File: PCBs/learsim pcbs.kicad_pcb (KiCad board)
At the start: 2 copper layers, 11 parts, among them U1 ESP32-C6-DEV-KIT-N8, U2 MAX7219, U3 MAX7219

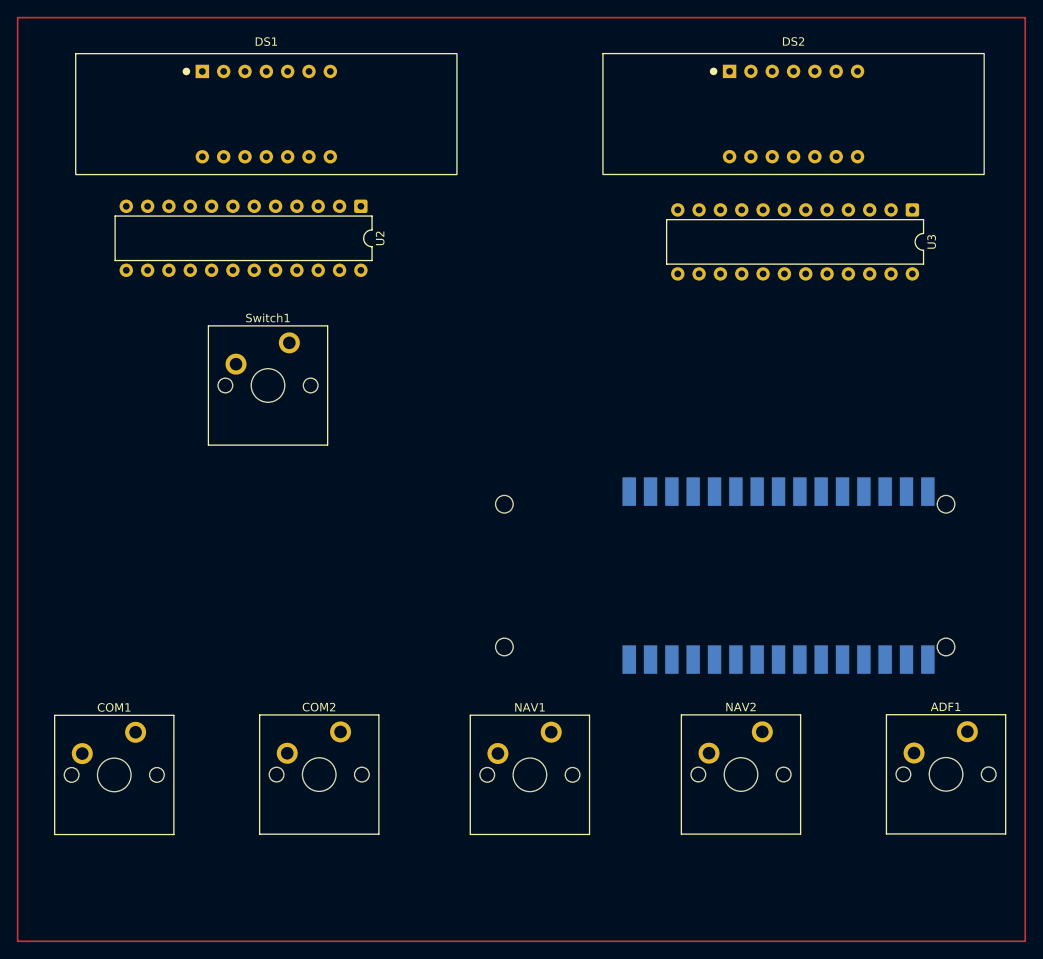
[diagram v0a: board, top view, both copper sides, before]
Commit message: pcb work
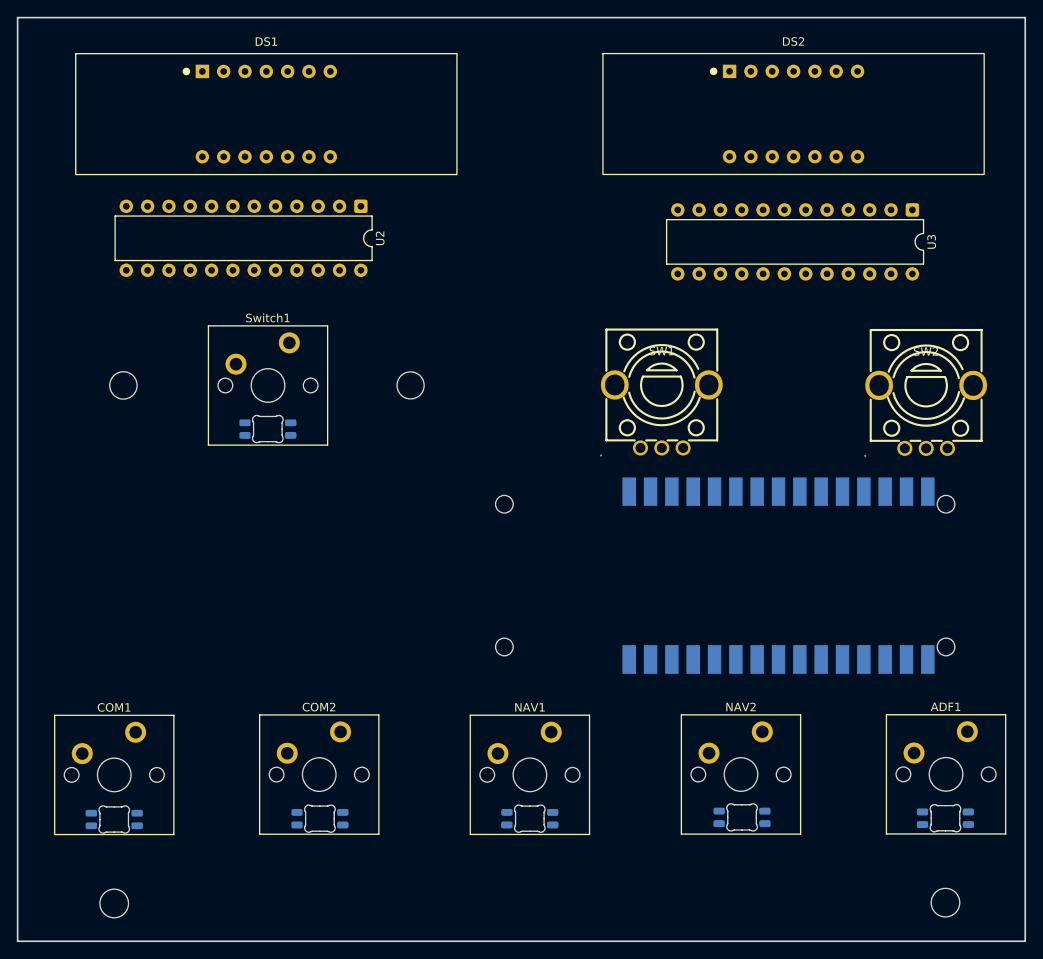
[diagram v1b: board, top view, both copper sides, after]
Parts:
- added D1: COM1, LED_SMD:LED_SK6812MINI-E_3.2x2.8mm_P1.5mm_ReverseMount, B.Cu at (32.5, 120.5)
- added D2: COM2, LED_SMD:LED_SK6812MINI-E_3.2x2.8mm_P1.5mm_ReverseMount, B.Cu at (57.0, 120.4)
- added D3: NAV1, LED_SMD:LED_SK6812MINI-E_3.2x2.8mm_P1.5mm_ReverseMount, B.Cu at (82.0, 120.4)
- added D4: NAV2, LED_SMD:LED_SK6812MINI-E_3.2x2.8mm_P1.5mm_ReverseMount, B.Cu at (107.3, 120.2)
- added D5: Switch1, LED_SMD:LED_SK6812MINI-E_3.2x2.8mm_P1.5mm_ReverseMount, B.Cu at (50.8, 74.0)
- added D6: ADF1, LED_SMD:LED_SK6812MINI-E_3.2x2.8mm_P1.5mm_ReverseMount, B.Cu at (131.5, 120.3)
- added SW1: MHz, Rotary:SW-TH_EC12EXXXX, F.Cu at (97.7, 72.5)
- added SW2: KHz, Rotary:SW-TH_EC12EXXXX, F.Cu at (129.2, 72.5)
- U1: footprint esppico:ESP32-C6-Pico -> ESP32-Pico:ESP32-C6-Pico
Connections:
- U1 pad 13: unconnected-(U1-GPIO21-Pad13) -> Net-(D1-DIN)
- U1 pad 16: unconnected-(U1-Vbus-Pad16) -> +5V
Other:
- board outline added: 120 x 110 mm
